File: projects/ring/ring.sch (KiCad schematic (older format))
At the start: 38 parts, among them Q1 AOCA32116E, U1 STM32WB55CEU6TR, U2 LSM6DSO32TR, U3 ANT016008LCS2442MA2, U4 BQ297xy, U5 TPS62840DLCR, Y1 NX1612SA-32.000MHZ-CHP-CIS-3

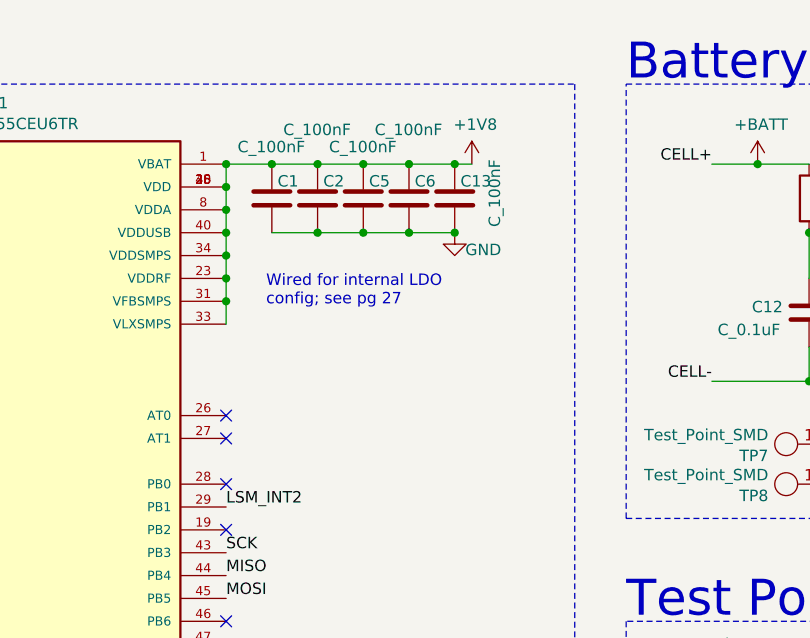
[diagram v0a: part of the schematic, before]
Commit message: just shipped first rev :fingers_crossed:
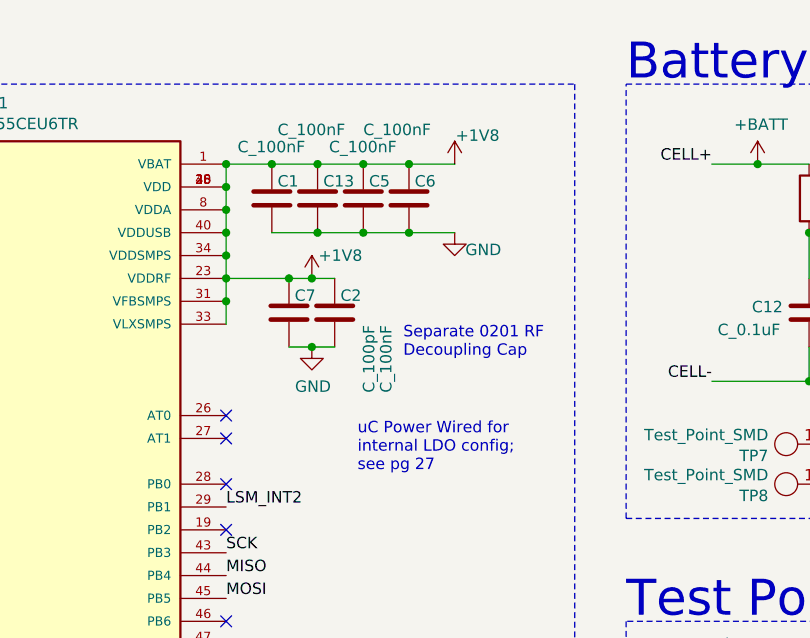
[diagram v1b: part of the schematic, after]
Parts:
- added C7: C_100pF, Capacitor_SMD:C_0201_0603Metric, symbol step:C_100pF
- C2: footprint Capacitor_SMD:C_0402_1005Metric -> Capacitor_SMD:C_0201_0603Metric
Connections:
- net +1V8: now also C7.1
- net GND: now also C7.2
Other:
- note added: "Separate 0201 RF \nDecoupling Cap\n"
- note added: "uC Power Wired for\ninternal LDO config; \nsee pg 27"
- note removed: "Wired for internal LDO \nconfig; see pg 27"
- moved on the sheet: C13, C2
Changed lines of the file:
@@
 encoding utf-8
 Sheet 1 1
-Title "RING_PCB"
+Title "RING PCB V0.0"
 Date "2022-04-06"
 Rev "REV1"
@@
 P 4600 1325
 F 0 "C6" H 4625 1400 50  0000 L CNN
-F 1 "C_100nF" H 4450 1625 50  0000 L CNN
+F 1 "C_100nF" H 4400 1625 50  0000 L CNN
 F 2 "Capacitor_SMD:C_0402_1005Metric" H 4638 1175 50  0001 C CNN
 F 3 "https://www.mouser.com/datasheet/2/212/KEM_C1002_X7R_SMD-1102033.pdf" H 4625 1425 50  0001 C CNN
@@
 L step:C_100nF C2
 U 1 1 625095B1
-P 4200 1325
-F 0 "C2" H 4225 1400 50  0000 L CNN
-F 1 "C_100nF" H 4050 1625 50  0000 L CNN
-F 2 "Capacitor_SMD:C_0402_1005Metric" H 4238 1175 50  0001 C CNN
-F 3 "https://www.mouser.com/datasheet/2/212/KEM_C1002_X7R_SMD-1102033.pdf" H 4225 1425 50  0001 C CNN
-F 4 "KEMET" H 4200 1325 60  0001 C CNN "MFN"
-F 5 "C0402C104K9RACTU" H 4200 1325 60  0001 C CNN "MPN"
-F 6 "https://www.mouser.com/ProductDetail/KEMET/C0402C104K9RACTU?qs=DBJr%252BvBUjU5VnZSA4JeTzg%3D%3D" H 4625 1825 60  0001 C CNN "buy"
-	1    4200 1325
+P 4275 1825
+F 0 "C2" H 4300 1900 50  0000 L CNN
+F 1 "C_100nF" V 4500 1475 50  0000 L CNN
+F 2 "Capacitor_SMD:C_0201_0603Metric" H 4313 1675 50  0001 C CNN
+F 3 "https://www.mouser.com/datasheet/2/212/KEM_C1002_X7R_SMD-1102033.pdf" H 4300 1925 50  0001 C CNN
+F 4 "KEMET" H 4275 1825 60  0001 C CNN "MFN"
+F 5 "C0402C104K9RACTU" H 4275 1825 60  0001 C CNN "MPN"
+F 6 "https://www.mouser.com/ProductDetail/KEMET/C0402C104K9RACTU?qs=DBJr%252BvBUjU5VnZSA4JeTzg%3D%3D" H 4700 2325 60  0001 C CNN "buy"
+	1    4275 1825
 	1    0    0    -1
 $EndComp
@@
 Connection ~ 4600 1175
 Connection ~ 3800 1175
-$Comp
-L power:GND #PWR0107
-U 1 1 62515C16
-P 4800 1475
-F 0 "#PWR0107" H 4800 1225 50  0001 C CNN
-F 1 "GND" H 4925 1400 50  0000 C CNN
-F 2 "" H 4800 1475 50  0001 C CNN
-F 3 "" H 4800 1475 50  0001 C CNN
-	1    4800 1475
-	1    0    0    -1
-$EndComp
 Connection ~ 4600 1475
 $Comp
@@
 	-1   0    0    1
 $EndComp
-$Comp
-L step:C_0.1uF C12
-U 1 1 625C9CB0
-P 6350 1825
-F 0 "C12" H 6100 1850 50  0000 L CNN
-F 1 "C_0.1uF" H 5950 1750 50  0000 L CNN
-F 2 "Capacitor_SMD:C_0402_1005Metric" H 6388 1675 50  0001 C CNN
-F 3 "http://datasheets.avx.com/X7RDielectric.pdf" H 6375 1925 50  0001 C CNN
-F 4 "DK" H 6350 1825 60  0001 C CNN "MFN"
-F 5 "478-3352-1-ND" H 6350 1825 60  0001 C CNN "MPN"
-F 6 "https://www.digikey.com/products/en?keywords=478-3352-1-ND" H 6775 2325 60  0001 C CNN "PurchasingLink"
-	1    6350 1825
-	1    0    0    -1
-$EndComp
 Wire Wire Line
 	6600 1675 6825 1675
@@
 	6125 1175 6350 1175
 $Comp
-L power:+1V8 #PWR0120
-U 1 1 625FF412
-P 4875 1175
-F 0 "#PWR0120" H 4875 1025 50  0001 C CNN
-F 1 "+1V8" H 4890 1348 50  0000 C CNN
-F 2 "" H 4875 1175 50  0001 C CNN
-F 3 "" H 4875 1175 50  0001 C CNN
-	1    4875 1175
-	1    0    0    -1
-$EndComp
-$Comp
 L power:+1V8 #PWR0121
 U 1 1 6261D39A
@@
 NoConn ~ 3800 3675
 NoConn ~ 3800 3775
-$Comp
-L step:C_100nF C13
-U 1 1 625B50DD
-P 4800 1325
-F 0 "C13" H 4825 1400 50  0000 L CNN
-F 1 "C_100nF" V 4975 1200 50  0000 L CNN
-F 2 "Capacitor_SMD:C_0402_1005Metric" H 4838 1175 50  0001 C CNN
-F 3 "https://www.mouser.com/datasheet/2/212/KEM_C1002_X7R_SMD-1102033.pdf" H 4825 1425 50  0001 C CNN
-F 4 "KEMET" H 4800 1325 60  0001 C CNN "MFN"
-F 5 "C0402C104K9RACTU" H 4800 1325 60  0001 C CNN "MPN"
-F 6 "https://www.mouser.com/ProductDetail/KEMET/C0402C104K9RACTU?qs=DBJr%252BvBUjU5VnZSA4JeTzg%3D%3D" H 5225 1825 60  0001 C CNN "buy"
-	1    4800 1325
-	1    0    0    -1
-$EndComp
-Wire Wire Line
-	4600 1175 4800 1175
-Connection ~ 4800 1175
-Wire Wire Line
-	4800 1175 4875 1175
 Wire Wire Line
 	4600 1475 4800 1475
@@
 Connection ~ 3800 1575
 Connection ~ 3800 1475
-Text Notes 3975 1800 0    50   ~ 0
-Wired for internal LDO \nconfig; see pg 27
 Text Notes 975  1850 0    50   ~ 0
 32MHz External \nclk; required for RF
-Connection ~ 4800 1475
 Wire Wire Line
 	7625 1675 7975 1675
@@
 NoConn ~ 3800 2275
 NoConn ~ 3800 2375
+$Comp
+L step:C_0.1uF C12
+U 1 1 625C9CB0
+P 6350 1825
+F 0 "C12" H 6100 1850 50  0000 L CNN
+F 1 "C_0.1uF" H 5950 1750 50  0000 L CNN
+F 2 "Capacitor_SMD:C_0402_1005Metric" H 6388 1675 50  0001 C CNN
+F 3 "http://datasheets.avx.com/X7RDielectric.pdf" H 6375 1925 50  0001 C CNN
+F 4 "DK" H 6350 1825 60  0001 C CNN "MFN"
+F 5 "478-3352-1-ND" H 6350 1825 60  0001 C CNN "MPN"
+F 6 "https://www.digikey.com/products/en?keywords=478-3352-1-ND" H 6775 2325 60  0001 C CNN "PurchasingLink"
+	1    6350 1825
+	1    0    0    -1
+$EndComp
+Text Notes 4375 2525 0    50   ~ 0
+uC Power Wired for\ninternal LDO config; \nsee pg 27
+$Comp
+L power:GND #PWR0107
+U 1 1 62515C16
+P 4800 1475
+F 0 "#PWR0107" H 4800 1225 50  0001 C CNN
+F 1 "GND" H 4925 1400 50  0000 C CNN
+F 2 "" H 4800 1475 50  0001 C CNN
+F 3 "" H 4800 1475 50  0001 C CNN
+	1    4800 1475
+	1    0    0    -1
+$EndComp
+$Comp
+L power:+1V8 #PWR0120
+U 1 1 625FF412
+P 4800 1175
+F 0 "#PWR0120" H 4800 1025 50  0001 C CNN
+F 1 "+1V8" H 4900 1300 50  0000 C CNN
+F 2 "" H 4800 1175 50  0001 C CNN
+F 3 "" H 4800 1175 50  0001 C CNN
+	1    4800 1175
+	1    0    0    -1
+$EndComp
+$Comp
+L step:C_100nF C13
+U 1 1 625B50DD
+P 4200 1325
+F 0 "C13" H 4225 1400 50  0000 L CNN
+F 1 "C_100nF" H 4025 1625 50  0000 L CNN
+F 2 "Capacitor_SMD:C_0402_1005Metric" H 4238 1175 50  0001 C CNN
+F 3 "https://www.mouser.com/datasheet/2/212/KEM_C1002_X7R_SMD-1102033.pdf" H 4225 1425 50  0001 C CNN
+F 4 "KEMET" H 4200 1325 60  0001 C CNN "MFN"
+F 5 "C0402C104K9RACTU" H 4200 1325 60  0001 C CNN "MPN"
+F 6 "https://www.mouser.com/ProductDetail/KEMET/C0402C104K9RACTU?qs=DBJr%252BvBUjU5VnZSA4JeTzg%3D%3D" H 4625 1825 60  0001 C CNN "buy"
+	1    4200 1325
+	1    0    0    -1
+$EndComp
+$Comp
+L step:C_100pF C7
+U 1 1 625AAC09
+P 4075 1825
+F 0 "C7" H 4100 1900 50  0000 L CNN
+F 1 "C_100pF" V 4425 1475 50  0000 L CNN
+F 2 "Capacitor_SMD:C_0201_0603Metric" H 4113 1675 50  0001 C CNN
+F 3 "https://katalog.we-online.de/pbs/datasheet/885012007057.pdf" H 4100 1925 50  0001 C CNN
+F 4 "DK" H 4075 1825 60  0001 C CNN "MFN"
+F 5 "732-7852-1-ND" H 4075 1825 60  0001 C CNN "MPN"
+F 6 "https://www.digikey.com/product-detail/en/wurth-electronics-inc/885012007057/732-7852-1-ND/5454479" H 4500 2325 60  0001 C CNN "PurchasingLink"
+	1    4075 1825
+	1    0    0    -1
+$EndComp
+Wire Wire Line
+	3800 1675 4075 1675
+Wire Wire Line
+	4600 1175 4800 1175
+Connection ~ 4075 1675
+Wire Wire Line
+	4075 1675 4175 1675
+Wire Wire Line
+	4075 1975 4175 1975
+$Comp
+L power:GND #PWR03
+U 1 1 625BA310
+P 4175 1975
+F 0 "#PWR03" H 4175 1725 50  0001 C CNN
+F 1 "GND" H 4180 1802 50  0000 C CNN
+F 2 "" H 4175 1975 50  0001 C CNN
+F 3 "" H 4175 1975 50  0001 C CNN
+	1    4175 1975
+	1    0    0    -1
+$EndComp
+Connection ~ 4175 1975
+Wire Wire Line
+	4175 1975 4275 1975
+$Comp
+L power:+1V8 #PWR02
+U 1 1 625BA8F7
+P 4175 1675
+F 0 "#PWR02" H 4175 1525 50  0001 C CNN
+F 1 "+1V8" H 4300 1775 50  0000 C CNN
+F 2 "" H 4175 1675 50  0001 C CNN
+F 3 "" H 4175 1675 50  0001 C CNN
+	1    4175 1675
+	1    0    0    -1
+$EndComp
+Connection ~ 4175 1675
+Wire Wire Line
+	4175 1675 4275 1675
+Text Notes 4575 2025 0    50   ~ 0
+Separate 0201 RF \nDecoupling Cap\n
 $EndSCHEMATC
